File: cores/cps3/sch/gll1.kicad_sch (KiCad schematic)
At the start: 13 parts, among them J11 DL-3429-GLL1

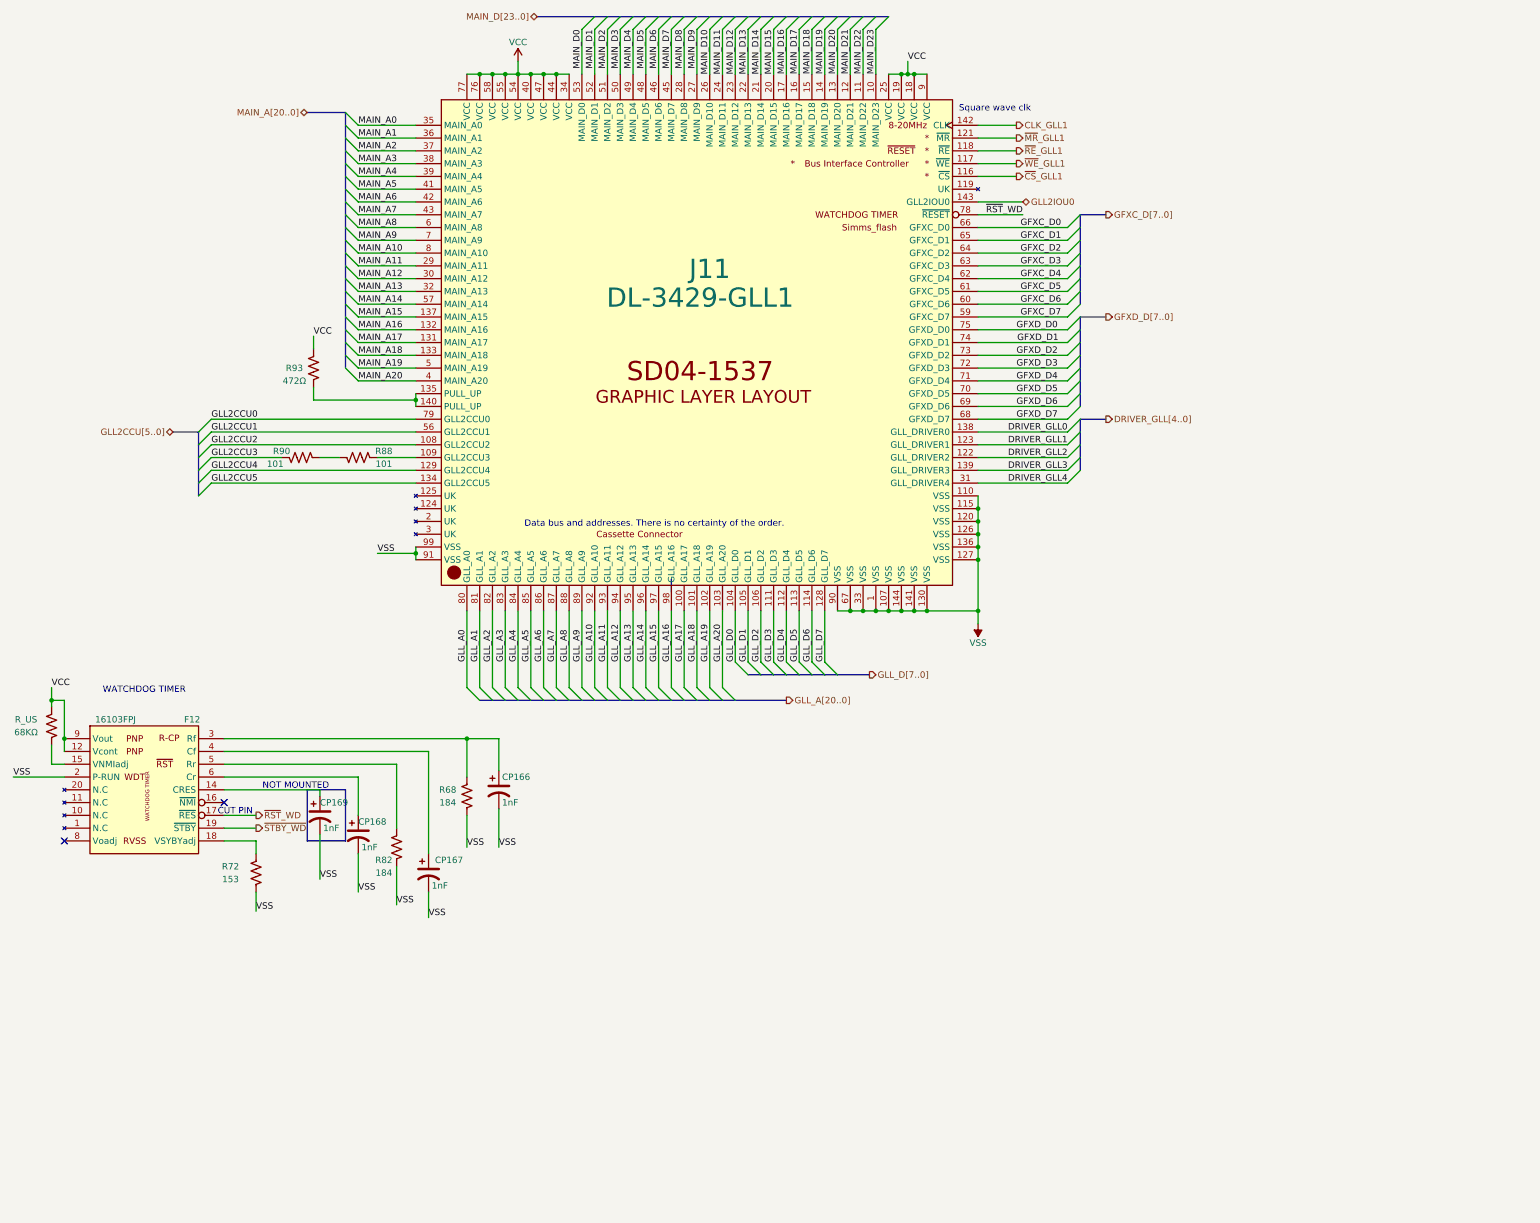
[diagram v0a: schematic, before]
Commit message: wip_cassette_sh2
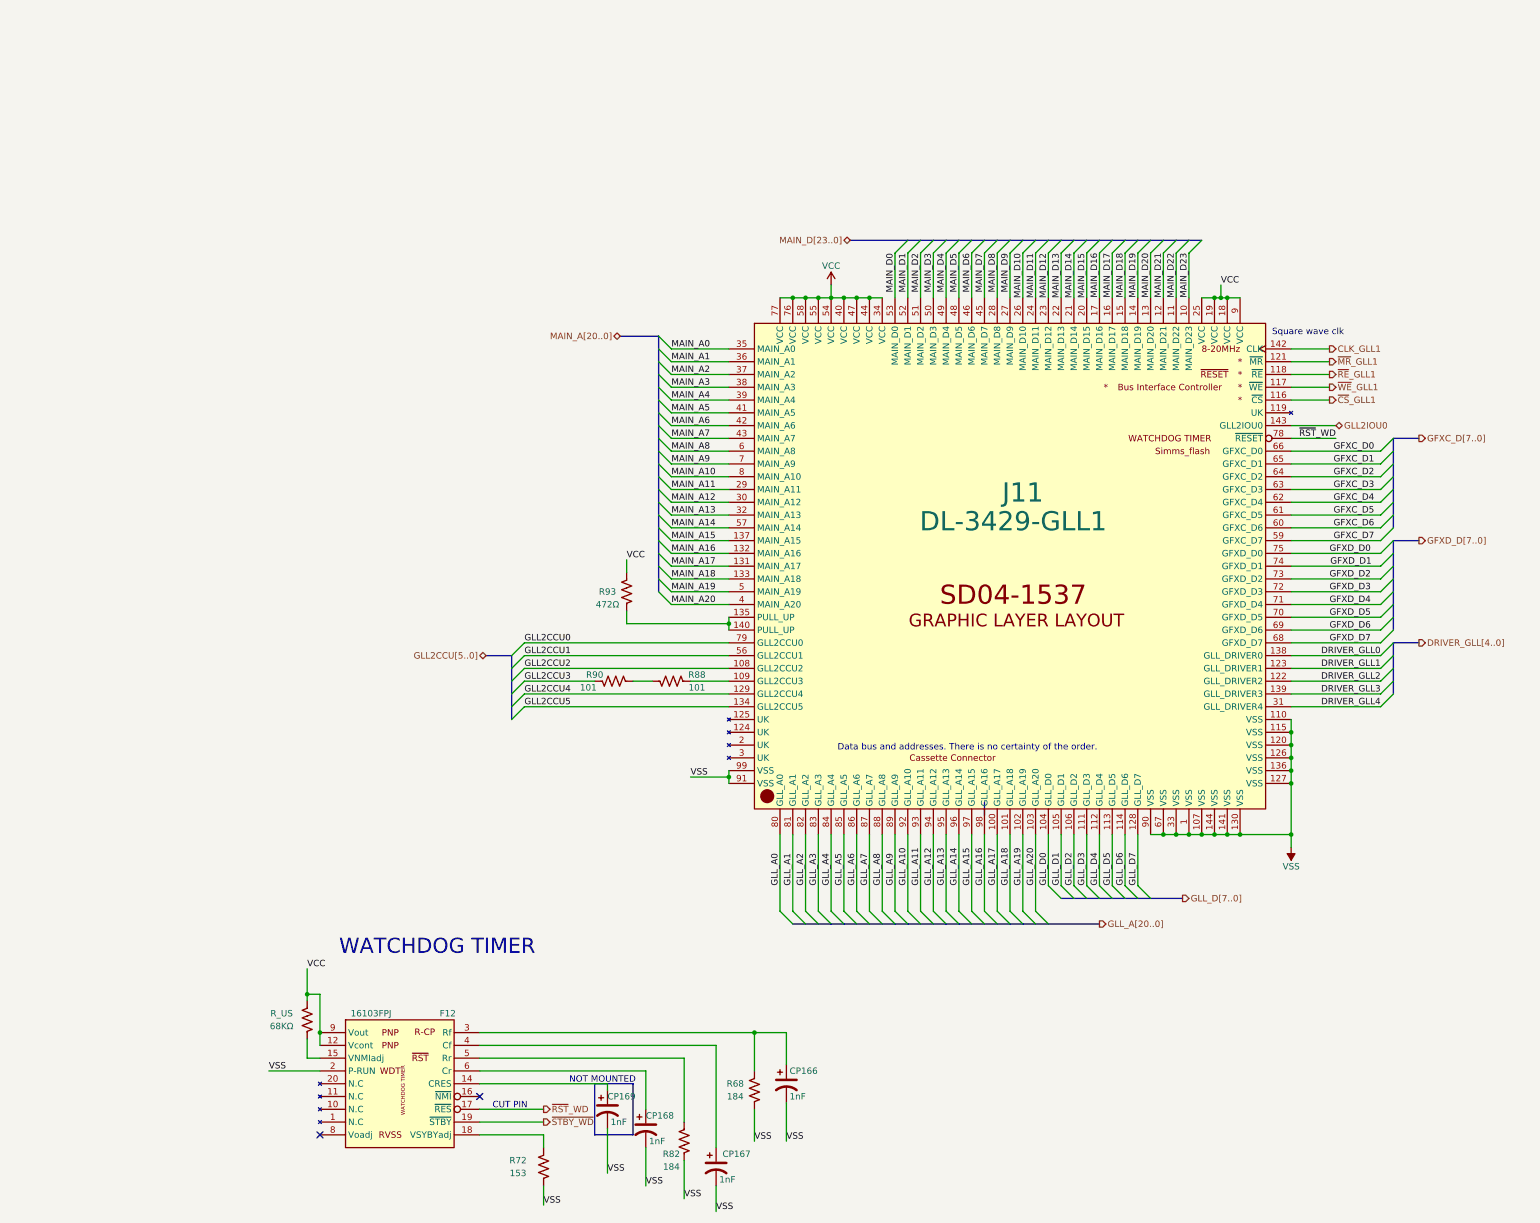
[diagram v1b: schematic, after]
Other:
- moved on the sheet: CP166, CP167, CP168, CP169, F12, J11, R68, R72, R82, R88, R90, R93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
